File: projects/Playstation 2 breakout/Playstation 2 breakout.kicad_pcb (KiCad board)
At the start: 2 copper layers, 35 x 40 mm, 11 parts

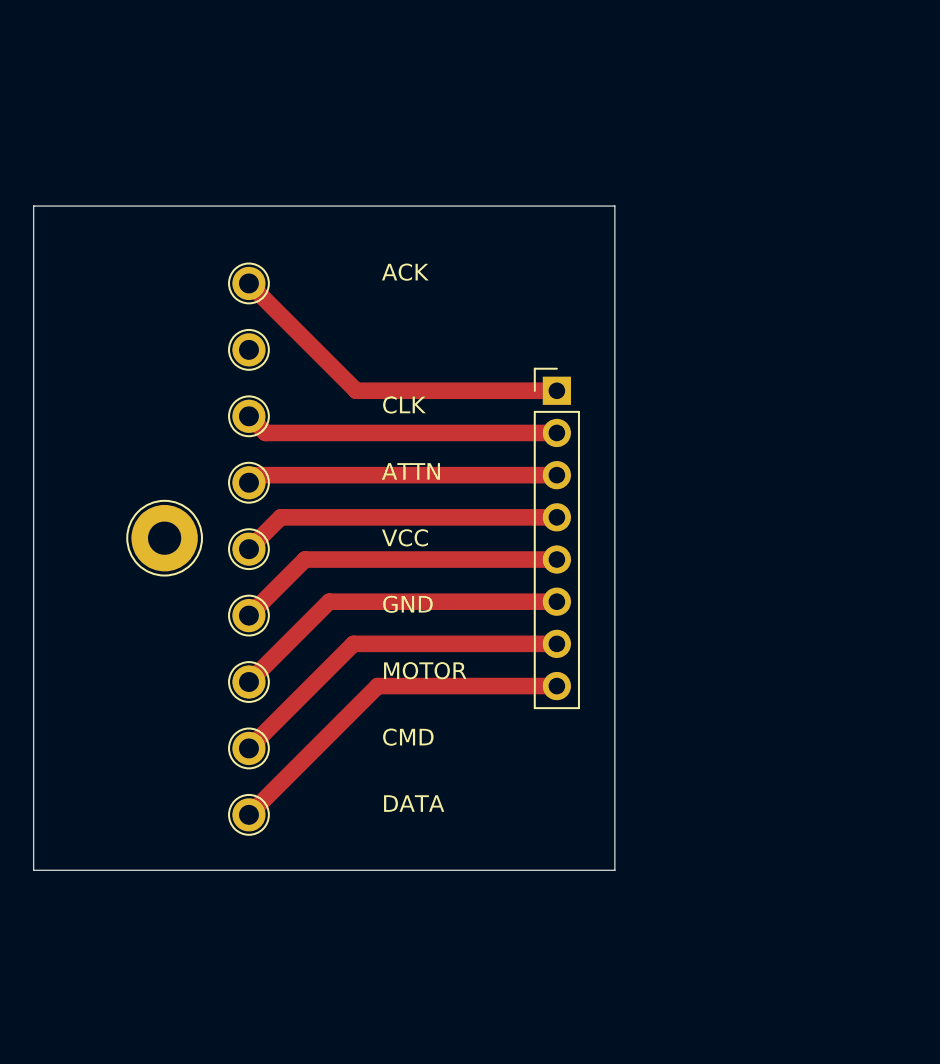
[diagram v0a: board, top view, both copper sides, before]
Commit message: updates
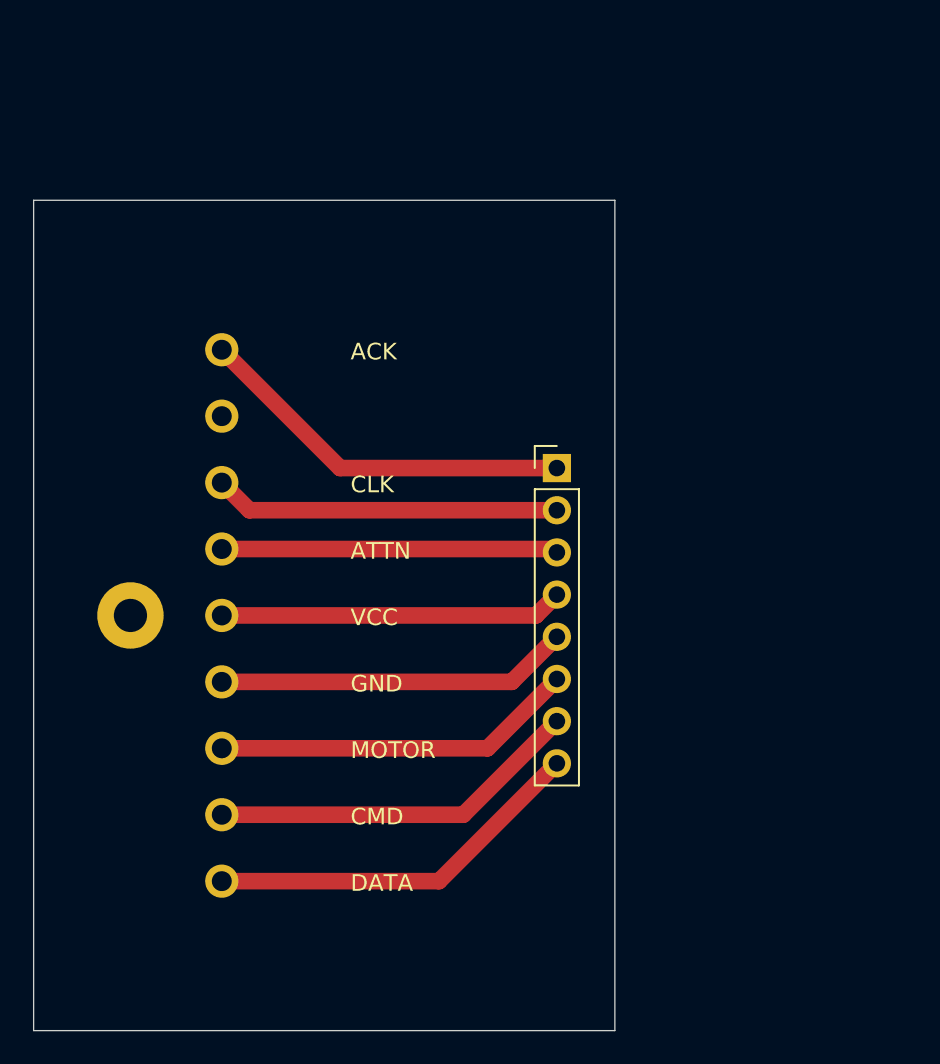
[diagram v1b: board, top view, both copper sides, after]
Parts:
- removed the REF** at (156.5, 78.1)
- removed the REF** at (156.5, 74.1)
- removed the REF** at (156.5, 94.1)
- removed the REF** at (156.5, 98.1)
- removed the REF** at (156.5, 90.1)
- removed the REF** at (156.5, 86.1)
- removed the REF** at (156.5, 66.1)
- removed the REF** at (151.4, 81.5)
- removed the REF** at (156.5, 70.1)
- removed the REF** at (156.5, 82.1)
- added REF**: Playstation 2 controller 180, Footprints_cez:Playstation 2 controller 180, F.Cu at (160.0, 82.8)
- moved REF** 4.65 mm to (175.0, 77.2)
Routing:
- net (no net): track 161.6 -> 173.8 mm
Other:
- board size 35 x 40 mm -> 35 x 50 mm
- board text removed: "ACK"
- board text removed: "ATTN"
- board text removed: "CLK"
- board text removed: "CMD"
- board text removed: "DATA"
- board text removed: "GND"
- board text removed: "MOTOR"
- board text removed: "VCC"

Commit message: and to the factory it goes
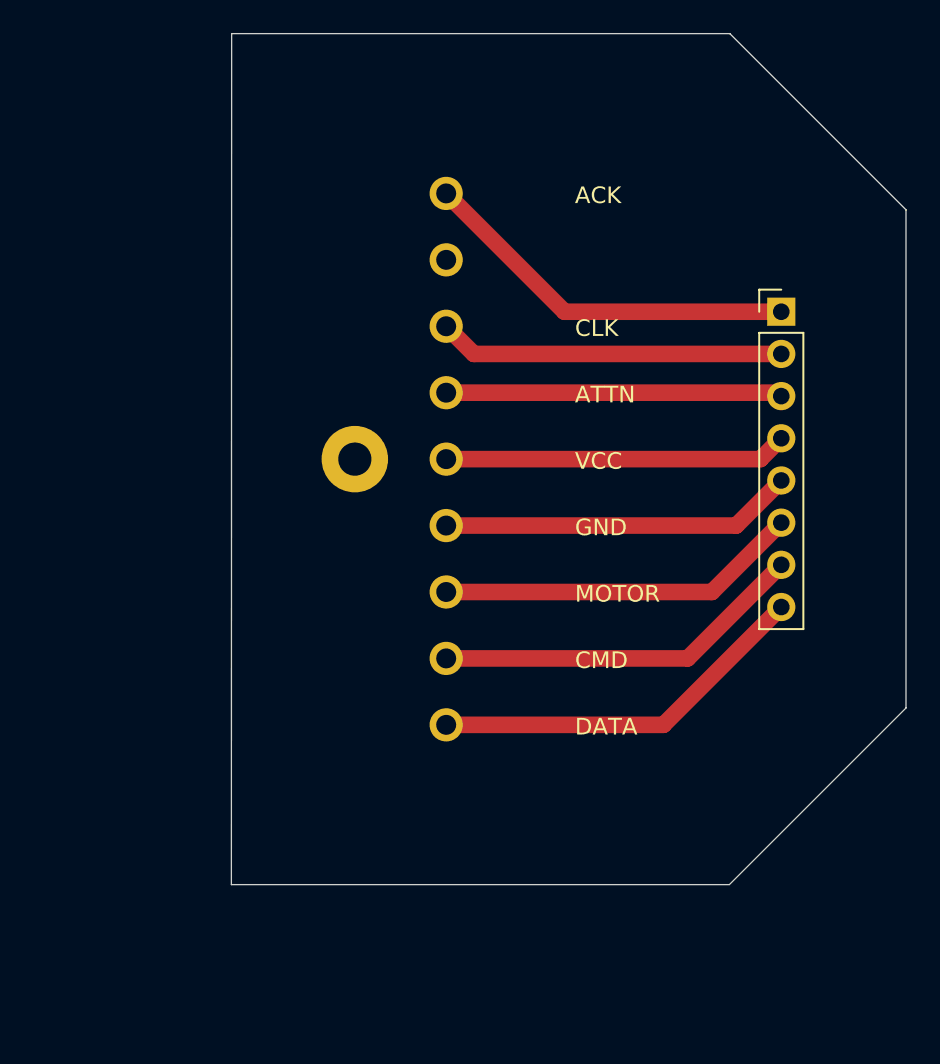
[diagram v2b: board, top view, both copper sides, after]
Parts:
- moved REF** 16.5 mm to (188.5, 67.8)
- moved REF** 16.5 mm to (173.5, 73.4)
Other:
- board size 35 x 50 mm -> 40.6 x 51.2 mm
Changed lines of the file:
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@@
 	(footprint "Footprints_cez:Playstation 2 controller 180"
 		(layer "F.Cu")
-		(at 160.02 82.804)
+		(at 173.5325 73.391)
 		(property "Reference" "REF**"
 			(at -5.952 -30.679625 0)
@@
 	(footprint "Connector_PinHeader_2.54mm:PinHeader_1x08_P2.54mm_Vertical"
 		(layer "F.Cu")
-		(at 175.004 77.246)
+		(at 188.5165 67.833)
 		(descr "Through hole straight pin header, 1x08, 2.54mm pitch, single row")
 		(tags "Through hole pin header THT 1x08 2.54mm single row")
@@
 		)
 	)
-	(gr_rect
-		(start 143.496 61.121)
-		(end 178.496 111.121)
+	(gr_line
+		(start 155.40335 102.329952)
+		(end 155.420049 51.086049)
 		(stroke
 			(width 0.05)
 			(type default)
 		)
-		(fill none)
 		(layer "Edge.Cuts")
 	)
-	(segment
-		(start 170.829 94.121)
-		(end 175.004 89.946)
-		(width 1)
-		(layer "F.Cu")
-		(net 0)
-	)
-	(segment
-		(start 174.799 82.121)
-		(end 175.004 82.326)
-		(width 1)
-		(layer "F.Cu")
-		(net 0)
-	)
-	(segment
-		(start 169.369 98.121)
-		(end 175.004 92.486)
-		(width 1)
-		(layer "F.Cu")
-		(net 0)
-	)
-	(segment
-		(start 156.491 79.786)
-		(end 175.004 79.786)
-		(width 1)
-		(layer "F.Cu")
-		(net 0)
-	)
-	(segment
-		(start 154.826 98.121)
-		(end 169.369 98.121)
-		(width 1)
-		(layer "F.Cu")
-		(net 0)
-	)
-	(segment
-		(start 154.826 78.121)
-		(end 156.491 79.786)
-		(width 1)
-		(layer "F.Cu")
-		(net 0)
-	)
-	(segment
-		(start 173.749 86.121)
-		(end 175.004 84.866)
-		(width 1)
-		(layer "F.Cu")
-		(net 0)
-	)
-	(segment
-		(start 154.826 94.121)
-		(end 170.829 94.121)
-		(width 1)
-		(layer "F.Cu")
-		(net 0)
-	)
-	(segment
-		(start 154.826 86.121)
-		(end 173.749 86.121)
-		(width 1)
-		(layer "F.Cu")
-		(net 0)
-	)
-	(segment
-		(start 172.289 90.121)
-		(end 175.004 87.406)
-		(width 1)
-		(layer "F.Cu")
-		(net 0)
-	)
-	(segment
-		(start 154.826 90.121)
-		(end 172.289 90.121)
-		(width 1)
-		(layer "F.Cu")
-		(net 0)
-	)
-	(segment
-		(start 161.951 77.246)
-		(end 175.004 77.246)
-		(width 1)
-		(layer "F.Cu")
-		(net 0)
-	)
-	(segment
-		(start 154.826 102.121)
-		(end 167.909 102.121)
-		(width 1)
-		(layer "F.Cu")
-		(net 0)
-	)
-	(segment
-		(start 154.826 70.121)
-		(end 161.951 77.246)
-		(width 1)
-		(layer "F.Cu")
-		(net 0)
-	)
-	(segment
-		(start 167.909 102.121)
-		(end 175.004 95.026)
-		(width 1)
-		(layer "F.Cu")
-		(net 0)
-	)
-	(segment
-		(start 154.826 82.121)
-		(end 174.799 82.121)
+	(gr_line
+		(start 185.40335 102.329952)
+		(end 155.40335 102.329952)
+		(stroke
+			(width 0.05)
+			(type default)
+		)
+		(layer "Edge.Cuts")
+	)
+	(gr_line
+		(start 185.420049 102.299253)
+		(end 196.026651 91.692651)
+		(stroke
+			(width 0.05)
+			(type default)
+		)
+		(layer "Edge.Cuts")
+	)
+	(gr_line
+		(start 196.026651 61.692651)
+		(end 185.420049 51.086049)
+		(stroke
+			(width 0.05)
+			(type default)
+		)
+		(layer "Edge.Cuts")
+	)
+	(gr_line
+		(start 185.420049 51.086049)
+		(end 155.420049 51.086049)
+		(stroke
+			(width 0.05)
+			(type default)
+		)
+		(layer "Edge.Cuts")
+	)
+	(gr_line
+		(start 196.026651 91.692651)
+		(end 196.026651 61.692651)
+		(stroke
+			(width 0.05)
+			(type default)
+		)
+		(layer "Edge.Cuts")
+	)
+	(segment
+		(start 184.3415 84.708)
+		(end 188.5165 80.533)
+		(width 1)
+		(layer "F.Cu")
+		(net 0)
+	)
+	(segment
+		(start 188.3115 72.708)
+		(end 188.5165 72.913)
+		(width 1)
+		(layer "F.Cu")
+		(net 0)
+	)
+	(segment
+		(start 182.8815 88.708)
+		(end 188.5165 83.073)
+		(width 1)
+		(layer "F.Cu")
+		(net 0)
+	)
+	(segment
+		(start 170.0035 70.373)
+		(end 188.5165 70.373)
+		(width 1)
+		(layer "F.Cu")
+		(net 0)
+	)
+	(segment
+		(start 168.3385 88.708)
+		(end 182.8815 88.708)
+		(width 1)
+		(layer "F.Cu")
+		(net 0)
+	)
+	(segment
+		(start 168.3385 68.708)
+		(end 170.0035 70.373)
+		(width 1)
+		(layer "F.Cu")
+		(net 0)
+	)
+	(segment
+		(start 187.2615 76.708)
+		(end 188.5165 75.453)
+		(width 1)
+		(layer "F.Cu")
+		(net 0)
+	)
+	(segment
+		(start 168.3385 84.708)
+		(end 184.3415 84.708)
+		(width 1)
+		(layer "F.Cu")
+		(net 0)
+	)
+	(segment
+		(start 168.3385 76.708)
+		(end 187.2615 76.708)
+		(width 1)
+		(layer "F.Cu")
+		(net 0)
+	)
+	(segment
+		(start 185.8015 80.708)
+		(end 188.5165 77.993)
+		(width 1)
+		(layer "F.Cu")
+		(net 0)
+	)
+	(segment
+		(start 168.3385 80.708)
+		(end 185.8015 80.708)
+		(width 1)
+		(layer "F.Cu")
+		(net 0)
+	)
+	(segment
+		(start 175.4635 67.833)
+		(end 188.5165 67.833)
+		(width 1)
+		(layer "F.Cu")
+		(net 0)
+	)
+	(segment
+		(start 168.3385 92.708)
+		(end 181.4215 92.708)
+		(width 1)
+		(layer "F.Cu")
+		(net 0)
+	)
+	(segment
+		(start 168.3385 60.708)
+		(end 175.4635 67.833)
+		(width 1)
+		(layer "F.Cu")
+		(net 0)
+	)
+	(segment
+		(start 181.4215 92.708)
+		(end 188.5165 85.613)
+		(width 1)
+		(layer "F.Cu")
+		(net 0)
+	)
+	(segment
+		(start 168.3385 72.708)
+		(end 188.3115 72.708)
 		(width 1)
 		(layer "F.Cu")
@@
 		(members "febffc64-50ce-454a-b3e2-645a13d8d85d")
 	)
+	(group ""
+		(members "000a48aa-d47e-43cd-8630-35ab8f9ee854" "02e565b5-22d6-49e2-b3e1-b4683fe3ce39"
+			"10149138-6944-4765-8999-1fb1fdb22407" "1321e891-f1bc-4369-a08f-6c572875a655"
+			"273dfc81-5b8e-4445-af5d-4a10f6dc961c" "290d307f-1007-45d5-b9a7-cc2ca901ce92"
+			"33535160-1350-4efe-8017-3c0351aa9111" "40531c24-adeb-40a6-939f-958ad8c5f4f0"
+			"556d7efe-f3b3-472e-8e3d-486f5cf43f09" "55d9a1ad-f05c-4eb9-af4d-82defece75a6"
+			"60a3576c-b093-418c-ac32-d33ece48804b" "60f2e214-57d1-436a-a56d-b212d91fde4a"
+			"6560b3dc-fdb1-4118-bbd8-e5ee5044142d" "816fd48d-86d2-4efd-878f-cb8d676e4170"
+			"9dcdda37-d34d-49a0-b2fc-f8e041de9a3e" "ade53bbb-4f46-40e5-b622-9bae4126ac7e"
+			"d340fbc9-f8dd-407d-a2ba-19f88e4ce369" "fc091db6-ce9e-4e63-99e4-be6640805a05"
+		)
+	)
+	(group ""
+		(members "0007a979-b5fc-4b75-be6a-ee44a23f8266" "20e9589a-588a-48fb-8e07-5c103505f6e7"
+			"3572e40b-5a1e-4c15-ad21-cd385c8c4f6f" "785c9d0e-158b-46ff-b981-359c8f606704"
+			"902fc203-7dc2-4ae1-91a7-7be61fe5ef6d" "d2b3dfb0-30fa-4fd0-9aa3-2b02ab170341"
+		)
+	)
 )
